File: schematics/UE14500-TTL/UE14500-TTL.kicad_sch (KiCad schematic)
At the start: 6 parts, among them J1 Edge 1, J2 Edge 2

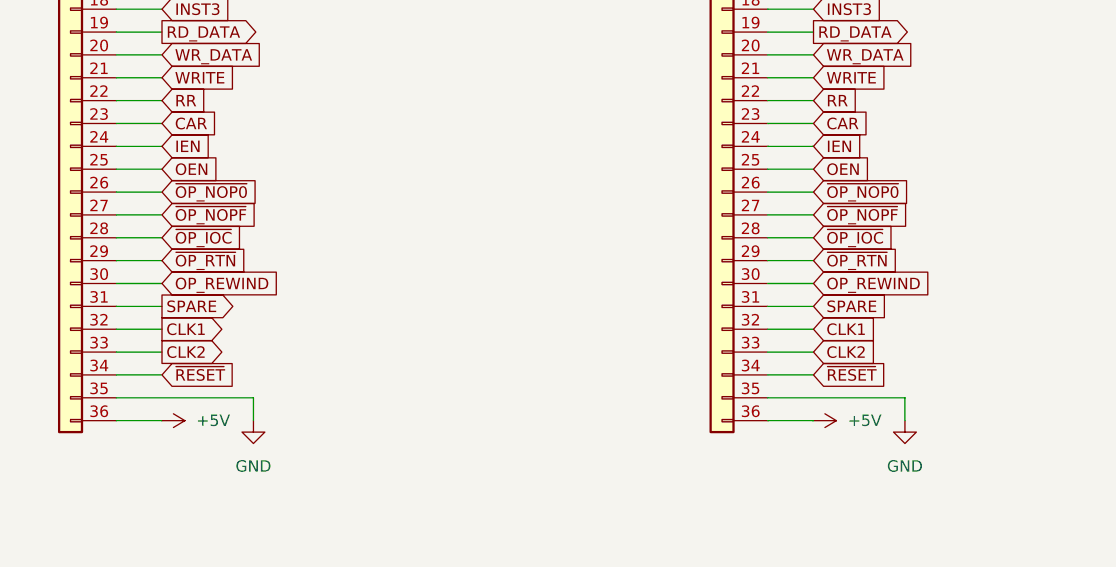
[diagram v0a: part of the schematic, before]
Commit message: Make some renderings of the computer
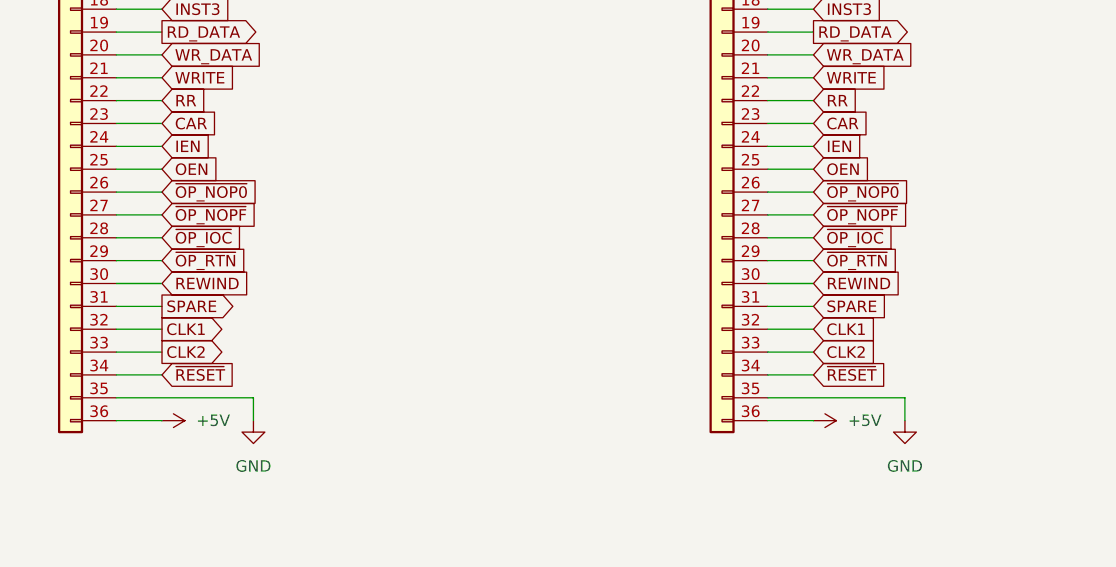
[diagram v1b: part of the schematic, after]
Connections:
- net OP_REWIND renamed REWIND
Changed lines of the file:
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@@
 		)
 	)
-	(global_label "OP_REWIND"
+	(global_label "REWIND"
 		(shape input)
 		(at 181.61 139.7 0)
@@
 		)
 		(property "Intersheetrefs" "${INTERSHEET_REFS}"
-			(at 195.239 139.7 0)
+			(at 191.6709 139.7 0)
 			(effects
 				(font
@@
 		)
 	)
-	(global_label "OP_REWIND"
+	(global_label "REWIND"
 		(shape input)
 		(at 109.22 139.7 0)
@@
 		)
 		(property "Intersheetrefs" "${INTERSHEET_REFS}"
-			(at 122.849 139.7 0)
-			(effects
-				(font
+			(at 119.2809 139.7 0)
+			(effects
+				(font

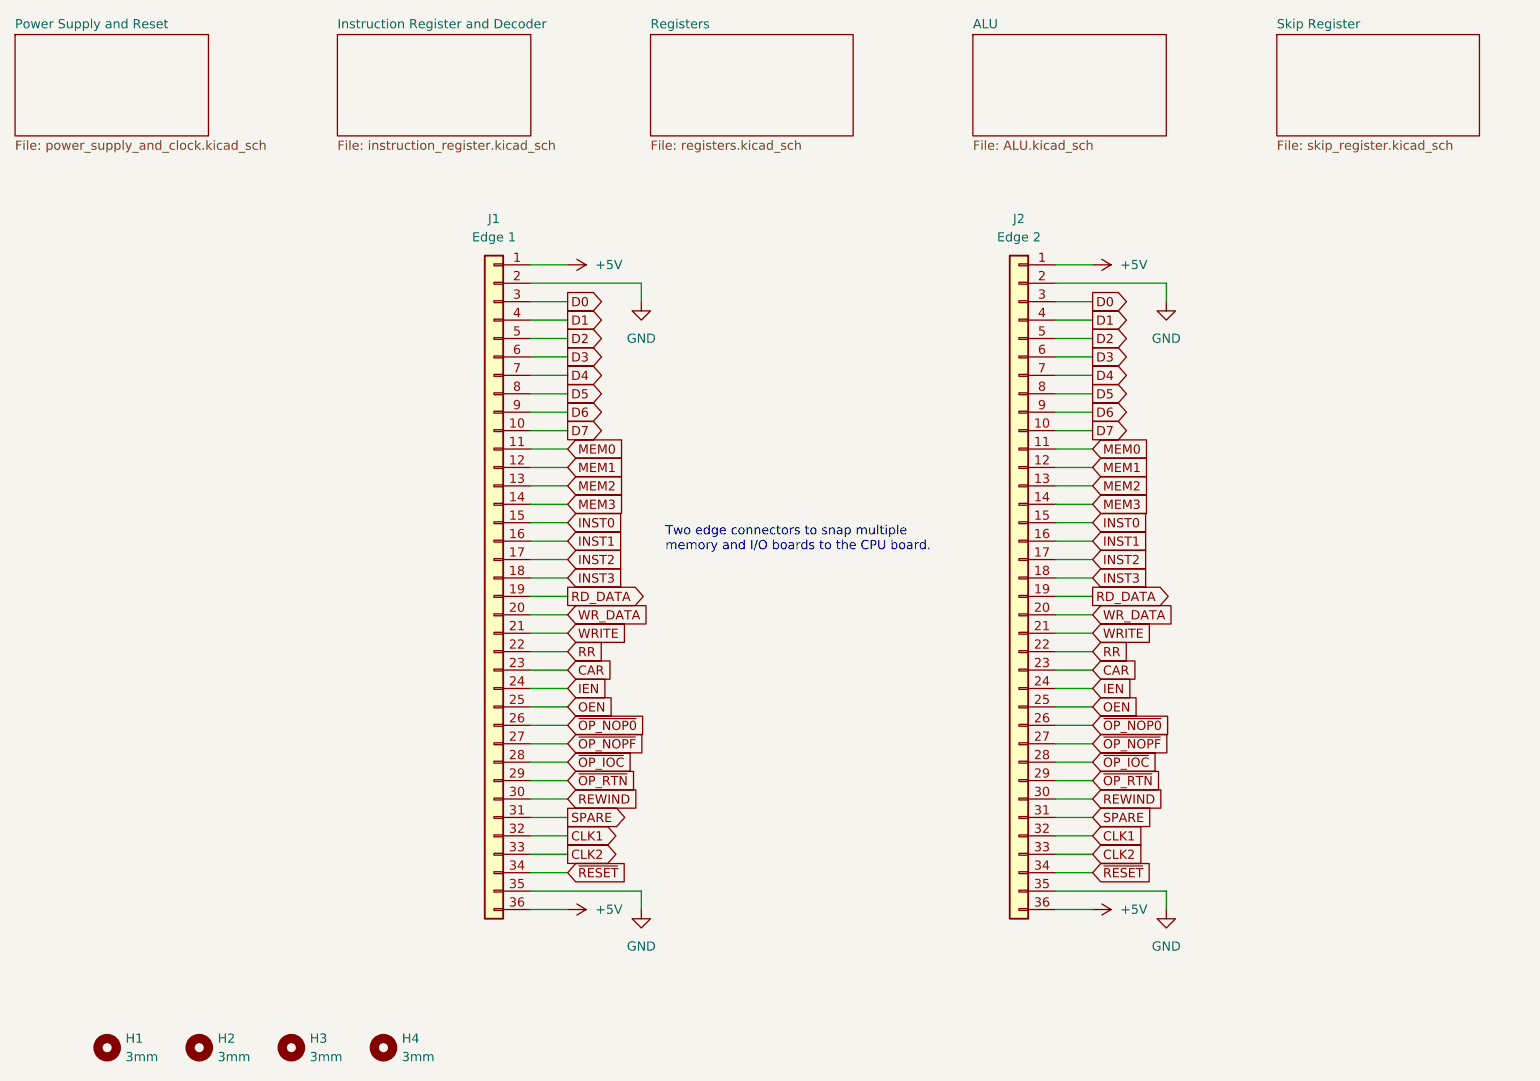
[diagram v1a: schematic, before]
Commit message: Lay out CPU board
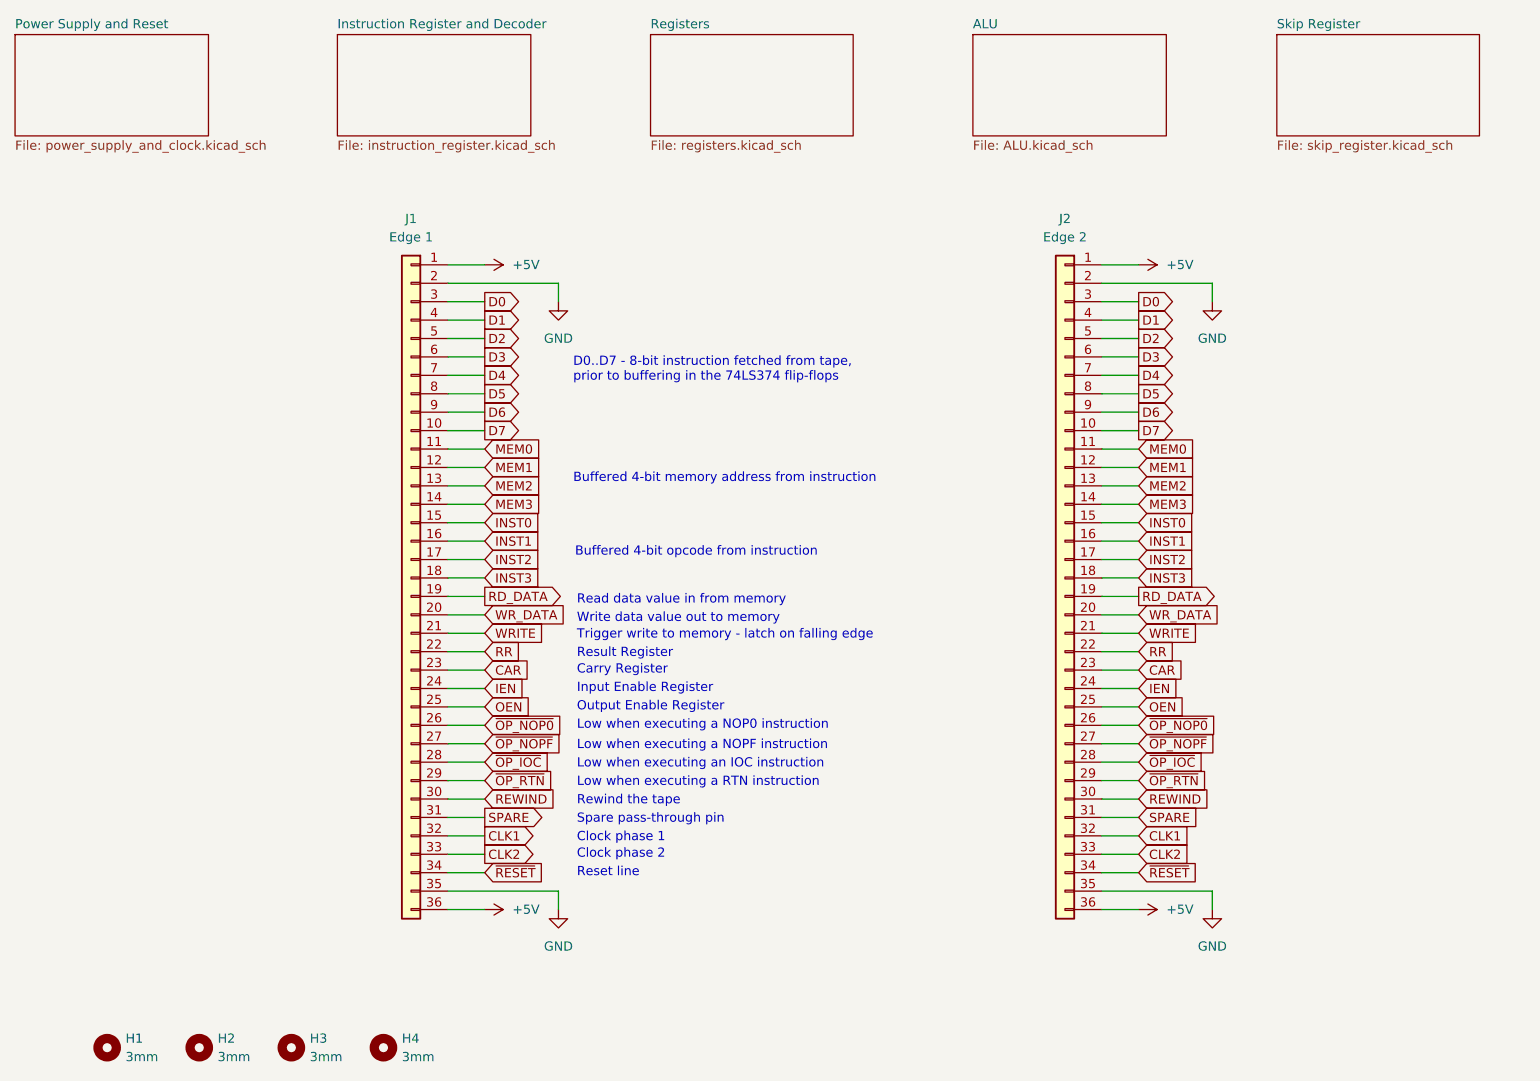
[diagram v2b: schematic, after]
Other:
- note added: "Buffered 4-bit memory address from instruction"
- note added: "Buffered 4-bit opcode from instruction"
- note added: "Carry Register"
- note added: "Clock phase 1"
- note added: "Clock phase 2"
- note added: "D0..D7 - 8-bit instruction fetched from tape, prior to buffering in the 74LS374 flip-flops"
- note added: "Input Enable Register"
- note added: "Low when executing a NOP0 instruction"
- note added: "Low when executing a NOPF instruction"
- note added: "Low when executing a RTN instruction"
- note added: "Low when executing an IOC instruction"
- note added: "Output Enable Register"
- note added: "Read data value in from memory"
- note added: "Reset line"
- note added: "Result Register"
- note added: "Rewind the tape"
- note added: "Spare pass-through pin"
- note added: "Trigger write to memory - latch on falling edge"
- note added: "Write data value out to memory"
- note removed: "Two edge connectors to snap multiple memory and I/O boards to the CPU board."
- moved on the sheet: J1, J2
